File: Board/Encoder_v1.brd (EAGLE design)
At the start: 89.6 x 106.3 mm, 22 parts, among them IC1 7805T, Q1 IRF640, Q2 IRF640, SW1 Encoder, X1 HD44780LCD-1602

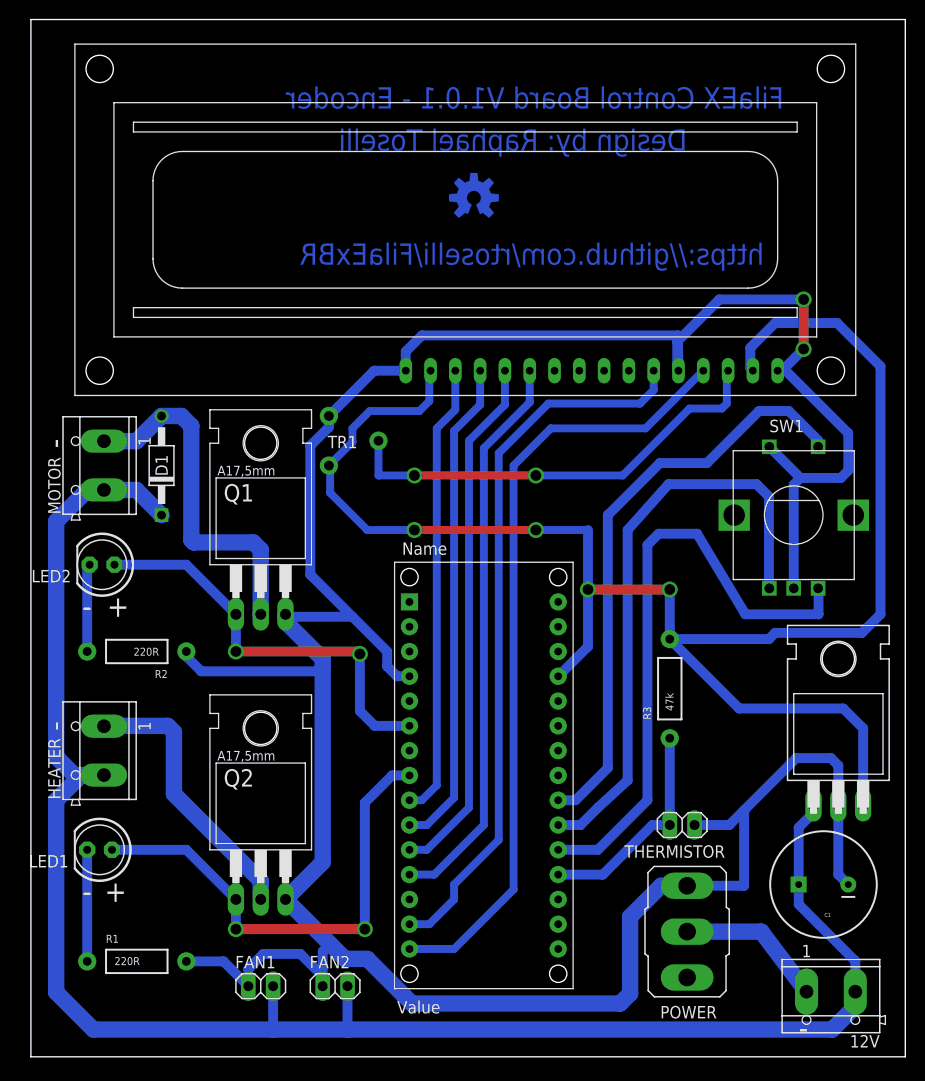
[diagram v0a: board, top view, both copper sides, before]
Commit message: Update board files and readme
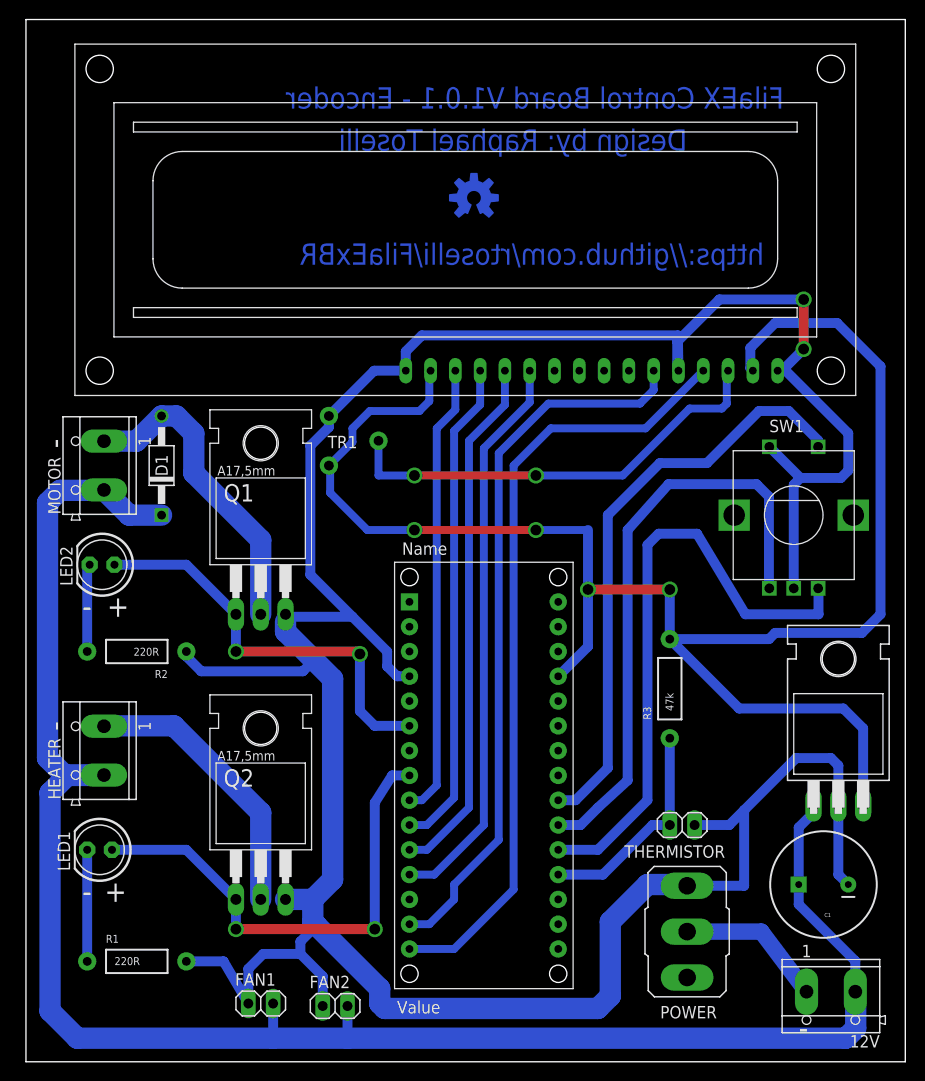
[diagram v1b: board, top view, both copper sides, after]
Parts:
- Q1, Q2: value IRF640 -> IRLB3813
- moved FAN2 2.03 mm to (31.8, 1.78)
- moved FAN1 1.78 mm to (24.1, 2.03)
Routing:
- net +12V: track 188.6 -> 196.1 mm
- net SWGND: track 315.8 -> 322.1 mm
- net N$12: track 36.9 -> 33.0 mm
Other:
- board size 89.6 x 106.3 mm -> 90.1 x 106.8 mm
